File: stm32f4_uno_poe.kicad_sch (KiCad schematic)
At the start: 13 parts, among them J101 STM32 GPIO, J102 Digital/PWM, J103 STM32 GPIO, J104 STM32 GPIO, J105 STM32 GPIO, J106 Power, J107 Conn_01x04, J108 Ethernet, J109 STM32 GPIO, J110 Digital/PWM, J111 Analog, J112 Barrel_Jack, J113 Conn_01x02

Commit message: #1 Use new central library KiCad-Lib
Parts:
- J113: footprint (none) -> Connector_PinHeader_2.54mm:PinHeader_1x02_P2.54mm_Vertical
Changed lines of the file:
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@@
       (effects (font (size 1.27 1.27)) (justify left))
     )
-    (property "Footprint" "" (at 128.27 57.15 0)
+    (property "Footprint" "Connector_PinHeader_2.54mm:PinHeader_1x02_P2.54mm_Vertical" (at 128.27 57.15 0)
       (effects (font (size 1.27 1.27)) hide)
     )

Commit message: #1 Use new central library KiCad-Lib
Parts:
- J112: footprint Connector_BarrelJack:BarrelJack_CUI_PJ-102AH_Horizontal -> #Connector:CUI Devices PJ-102AH.pdf; symbol Connector:Barrel_Jack_Switch -> #Connector:CUI Devices PJ-102AH
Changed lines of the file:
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@@
     )
   )
-  (symbol (lib_id "Connector:Barrel_Jack_Switch") (at 52.07 77.47 0) (unit 1)
+  (symbol (lib_id "#Connector:CUI Devices PJ-102AH") (at 52.07 77.47 0) (unit 1)
     (in_bom no) (on_board yes) (dnp no) (fields_autoplaced)
     (property "Reference" "J112" (at 52.07 69.215 0)
@@
       (effects (font (size 1 1)))
     )
-    (property "Footprint" "Connector_BarrelJack:BarrelJack_CUI_PJ-102AH_Horizontal" (at 53.34 78.486 0)
-      (effects (font (size 1 1)) hide)
+    (property "Footprint" "#Connector:CUI Devices PJ-102AH.pdf" (at 53.34 78.486 0)
+      (effects (font (size 1.27 1.27)) hide)
     )
-    (property "Datasheet" "~" (at 53.34 78.486 0)
-      (effects (font (size 1 1)) hide)
+    (property "Datasheet" "${KIPRJMOD}/KiCad-Lib/#Connector.doc/CUI Devices PJ-102AH.pdf" (at 53.34 78.486 0)
+      (effects (font (size 1.27 1.27)) hide)
     )
     (property "Description" "" (at 52.07 77.47 0)

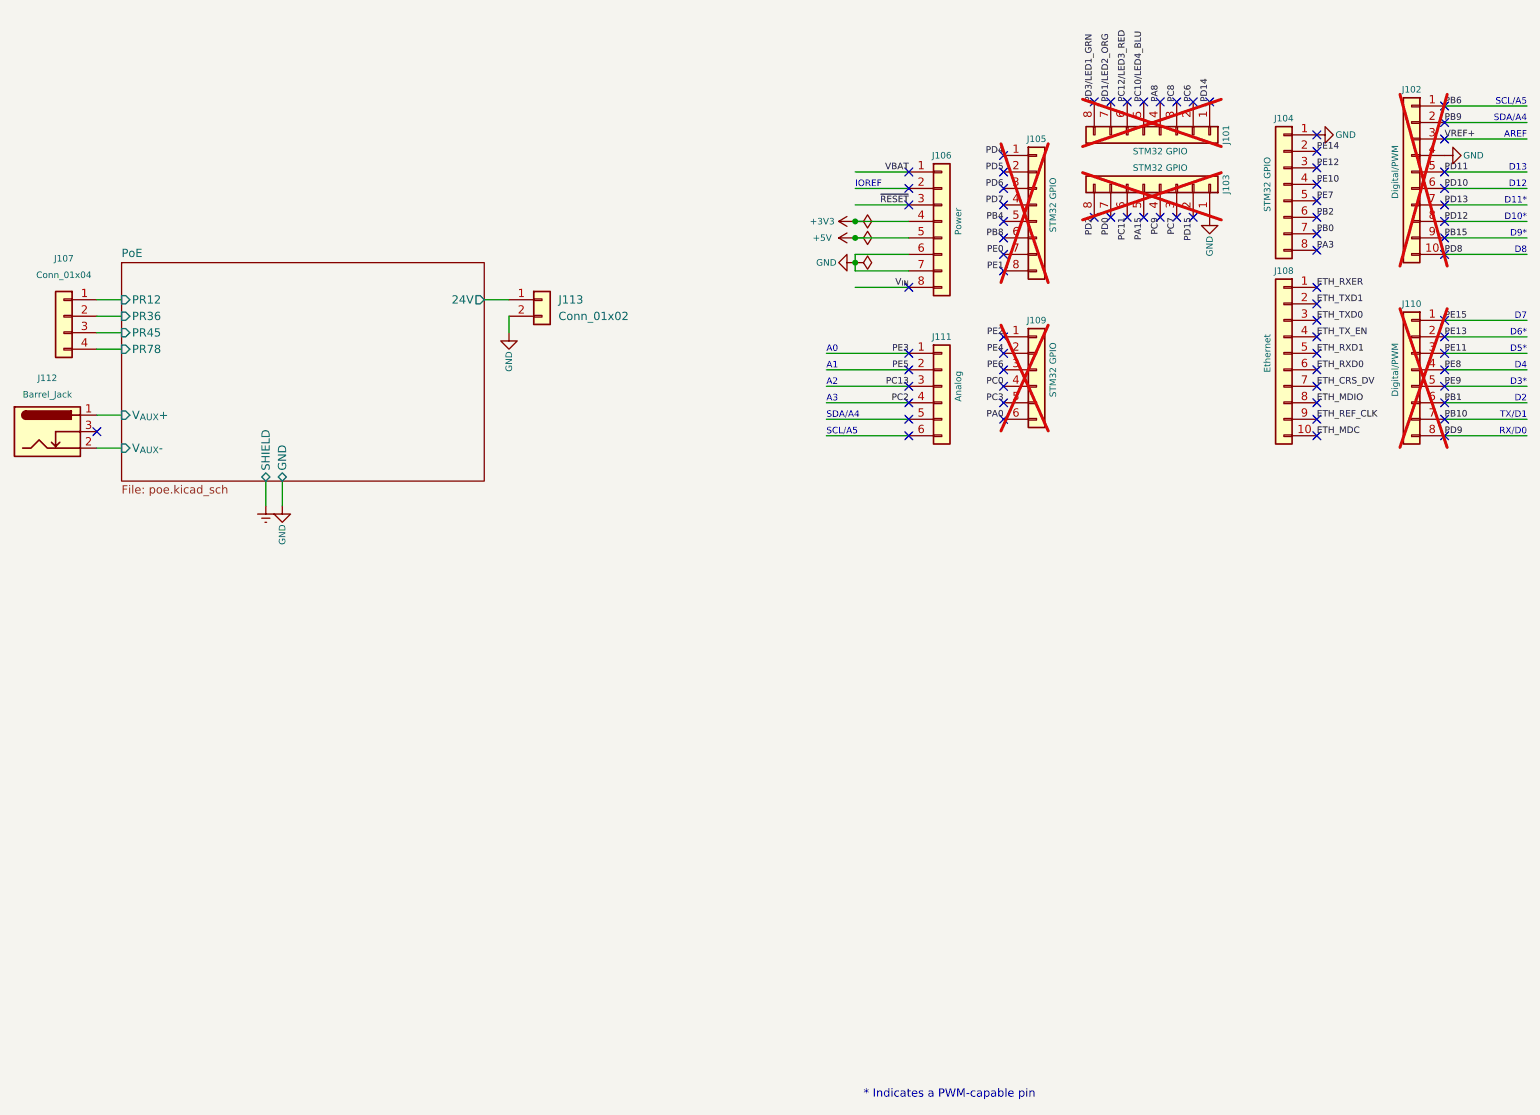
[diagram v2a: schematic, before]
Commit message: WIP
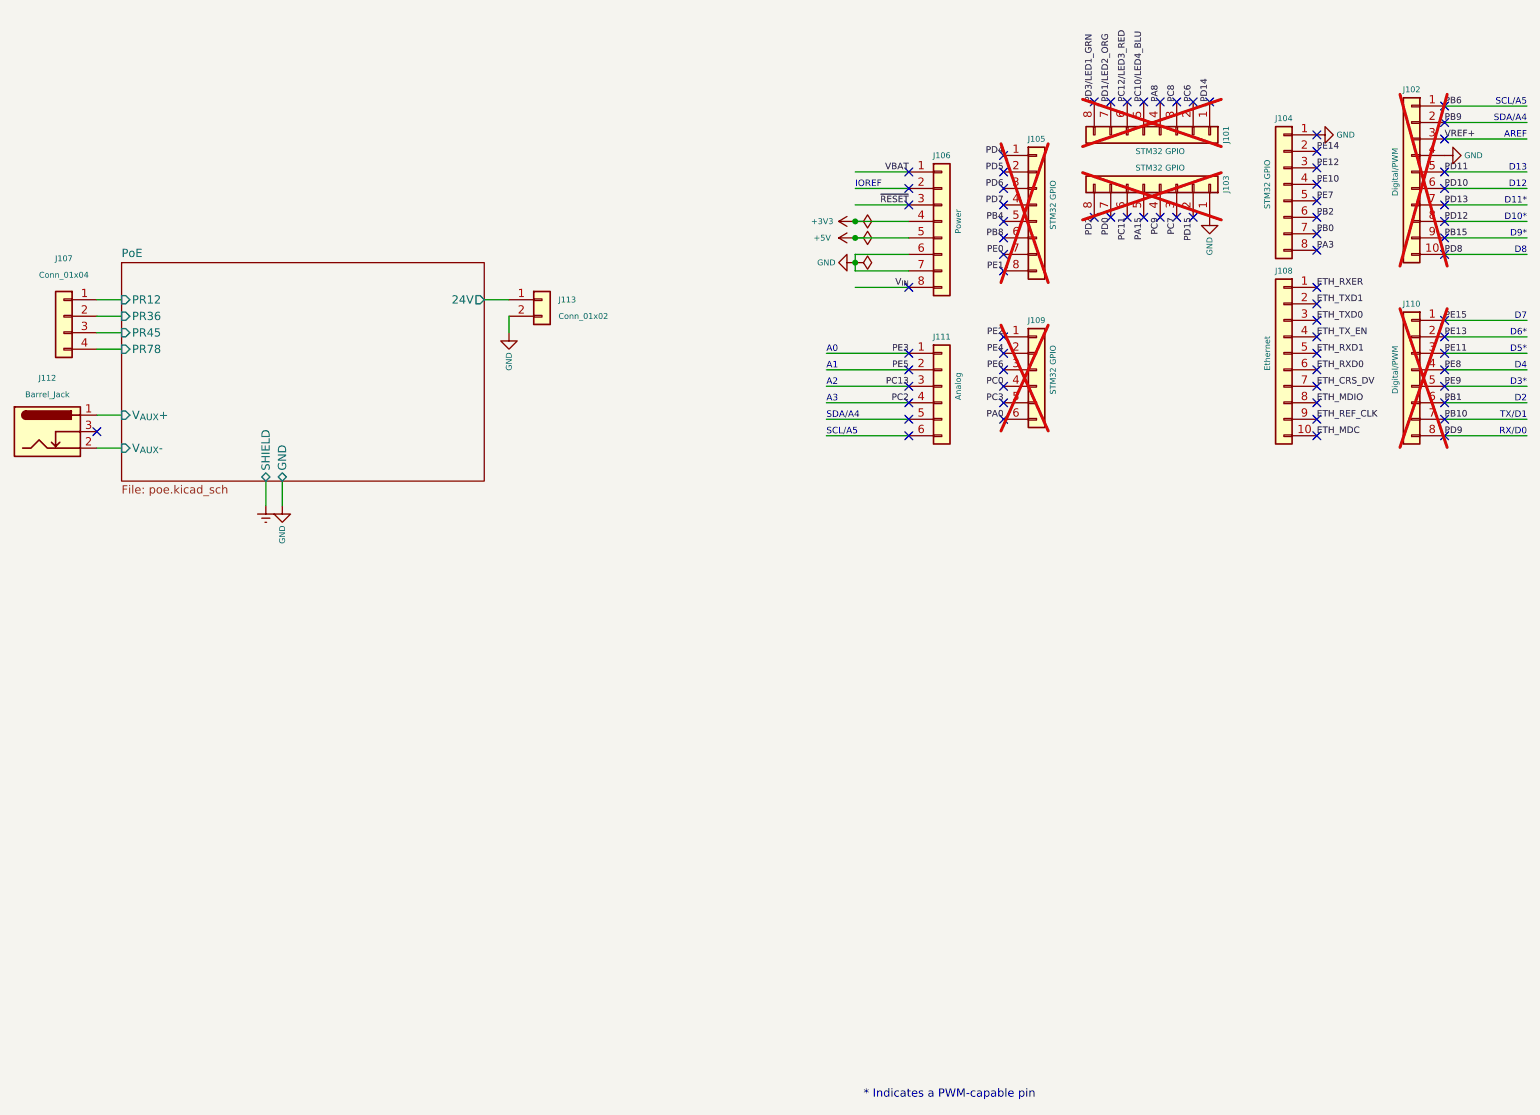
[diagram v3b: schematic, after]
